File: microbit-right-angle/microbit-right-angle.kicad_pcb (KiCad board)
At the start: 2 copper layers, 58.9 x 24.4 mm, 4 parts, among them J1 microbit_edge, J2 microbit_smd_socket

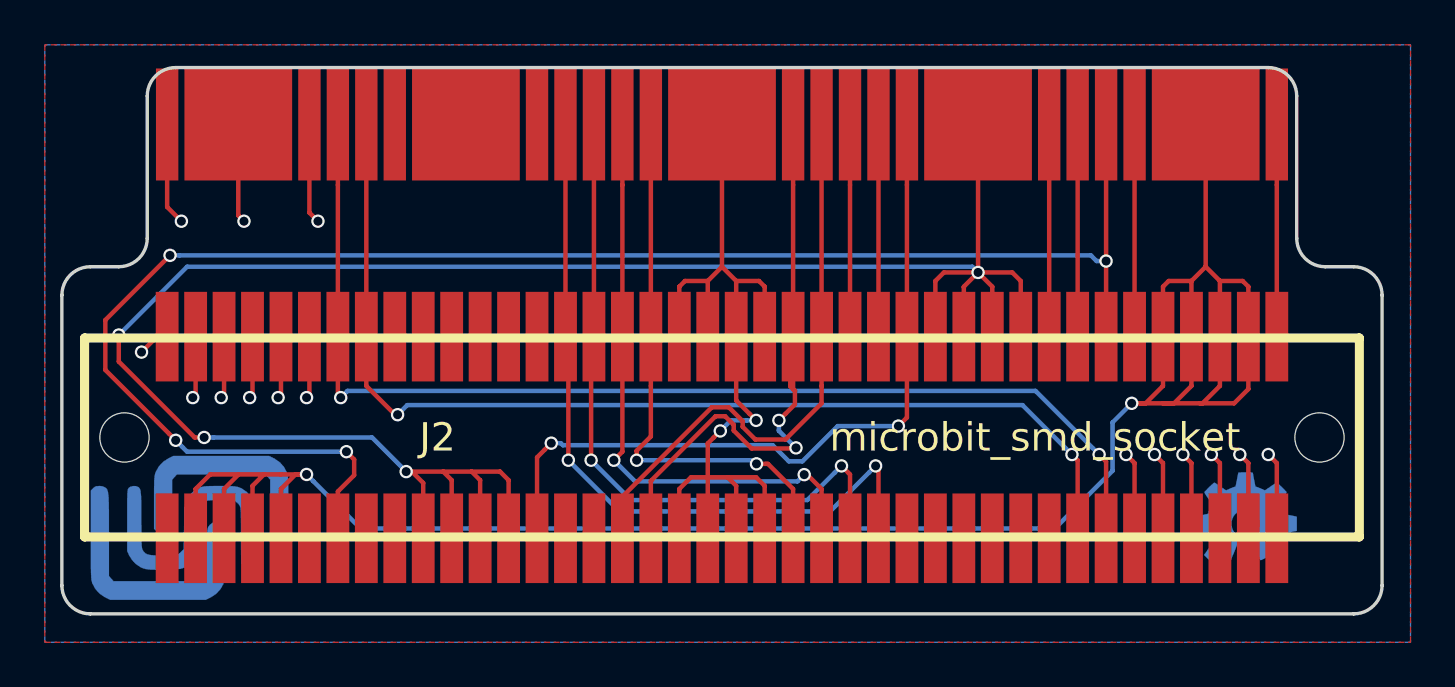
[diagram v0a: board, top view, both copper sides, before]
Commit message: Neaten up vias
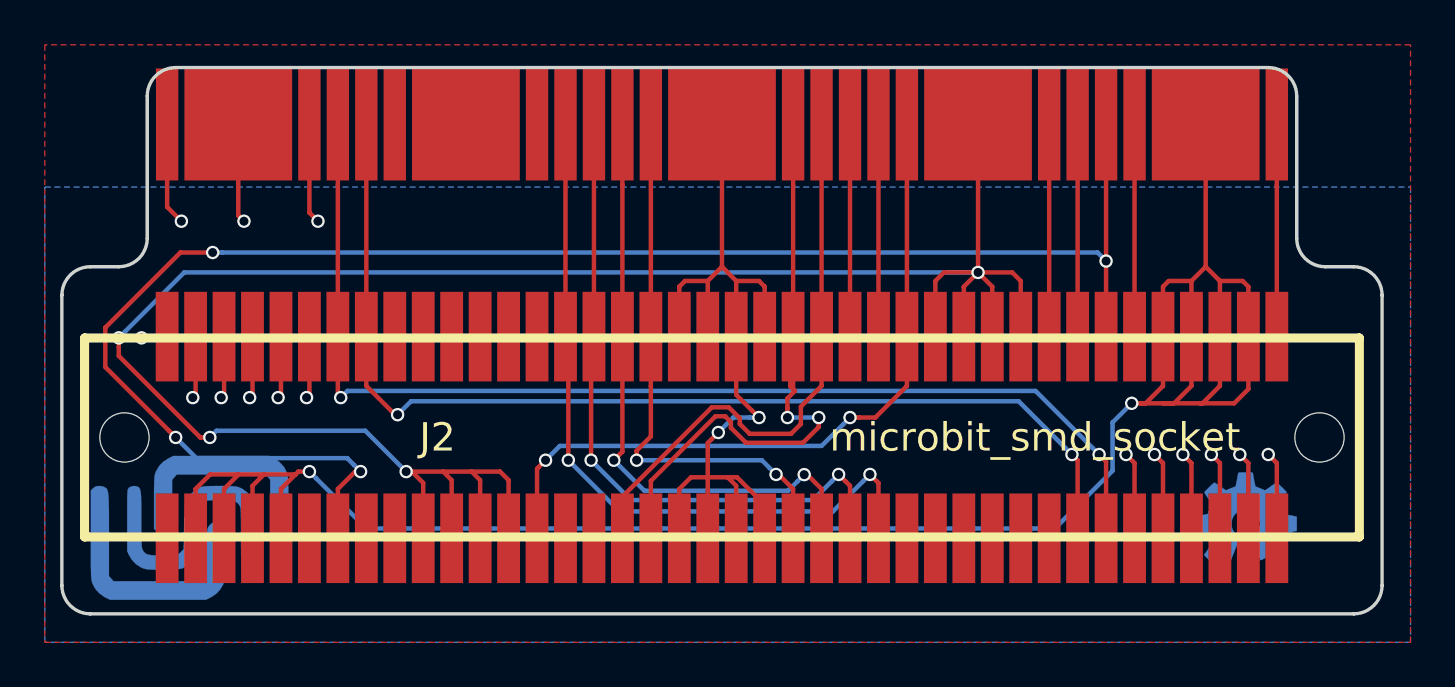
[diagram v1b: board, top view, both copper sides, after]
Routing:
- net MB_8: track 34.6 -> 32.8 mm
- net MB_12: track 28.5 -> 29.6 mm
- net MB_16: track 33.8 -> 33.1 mm
- net MB_15: track 31.0 -> 30.4 mm
